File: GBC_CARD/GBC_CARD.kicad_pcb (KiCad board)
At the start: 2 copper layers, 57.1 x 24 mm, 19 parts, among them J1 Conn_01x05_Pin, J2 GB_GBC_1x32, Q1 PMOS, Q2 BC817, U1 AW9523B, U2 AW9523B

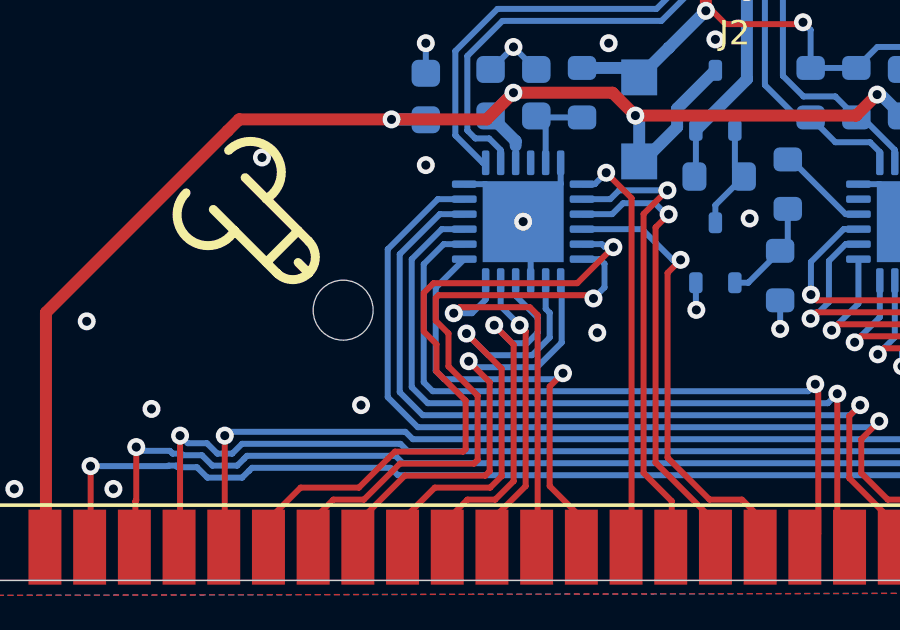
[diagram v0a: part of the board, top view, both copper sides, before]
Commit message: update pcb and upload schematic
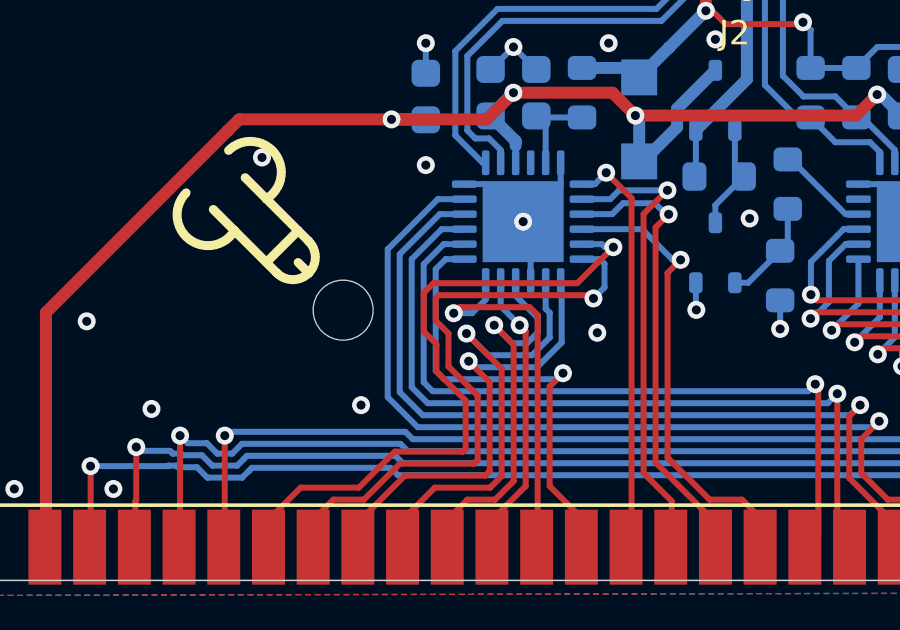
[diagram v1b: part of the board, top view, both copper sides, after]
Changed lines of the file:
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@@
 	)
 	(segment
-		(start 131.165 101.752)
-		(end 130.886 101.473)
-		(width 0.2)
-		(layer "B.Cu")
-		(net 21)
-	)
-	(segment
-		(start 130.886 98.701998)
+		(start 131.218686 97.75)
 		(end 131.837998 97.75)
 		(width 0.2)
@@
 	)
 	(segment
-		(start 130.886 101.473)
-		(end 130.886 98.701998)
+		(start 131.165 101.752)
+		(end 130.886 101.473)
 		(width 0.2)
 		(layer "B.Cu")
@@
 		(width 0.2)
 		(layer "B.Cu")
+		(net 21)
+	)
+	(segment
+		(start 130.886 101.473)
+		(end 130.886 98.082686)
+		(width 0.2)
+		(layer "B.Cu")
+		(net 21)
+	)
+	(segment
+		(start 130.886 98.082686)
+		(end 131.218686 97.75)
+		(width 0.2)
+		(layer "B.Cu")
